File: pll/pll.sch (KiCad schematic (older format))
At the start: 24 parts, among them SW1 SW_DIP_x05, U1 NE555, U2 74HC393, U3 74HC86, U4 LM7805, U5 NE555

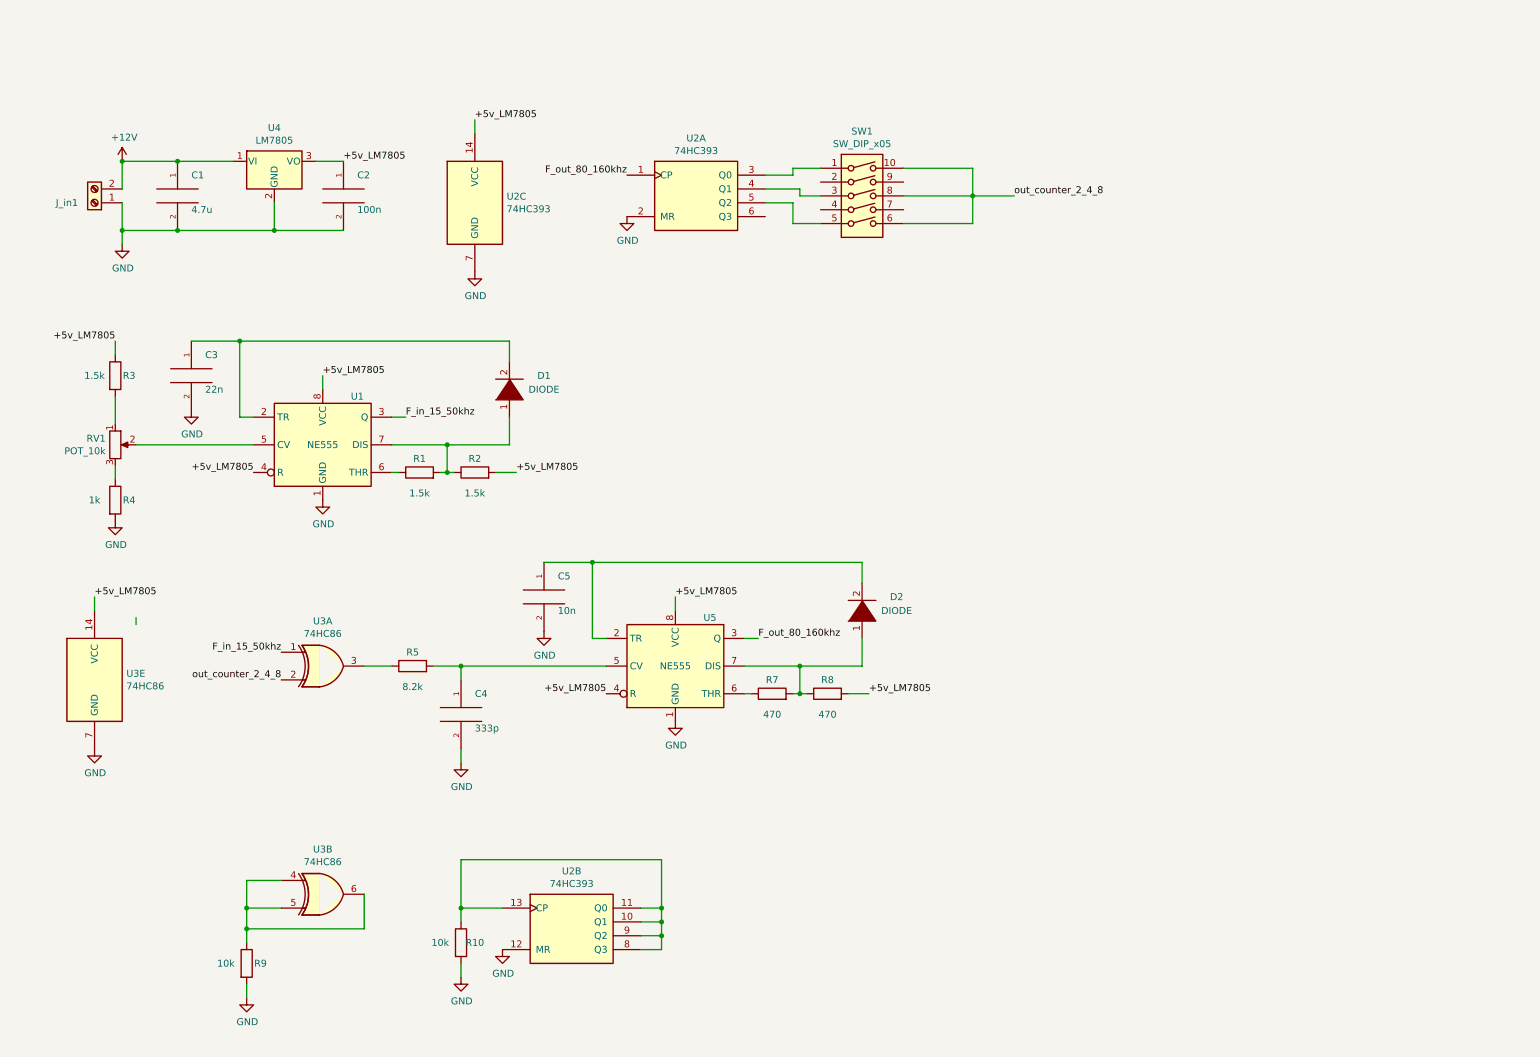
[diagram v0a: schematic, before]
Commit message: Update pll
Signed-off-by: Felipe Leon <fglfgl27@gmail.com>
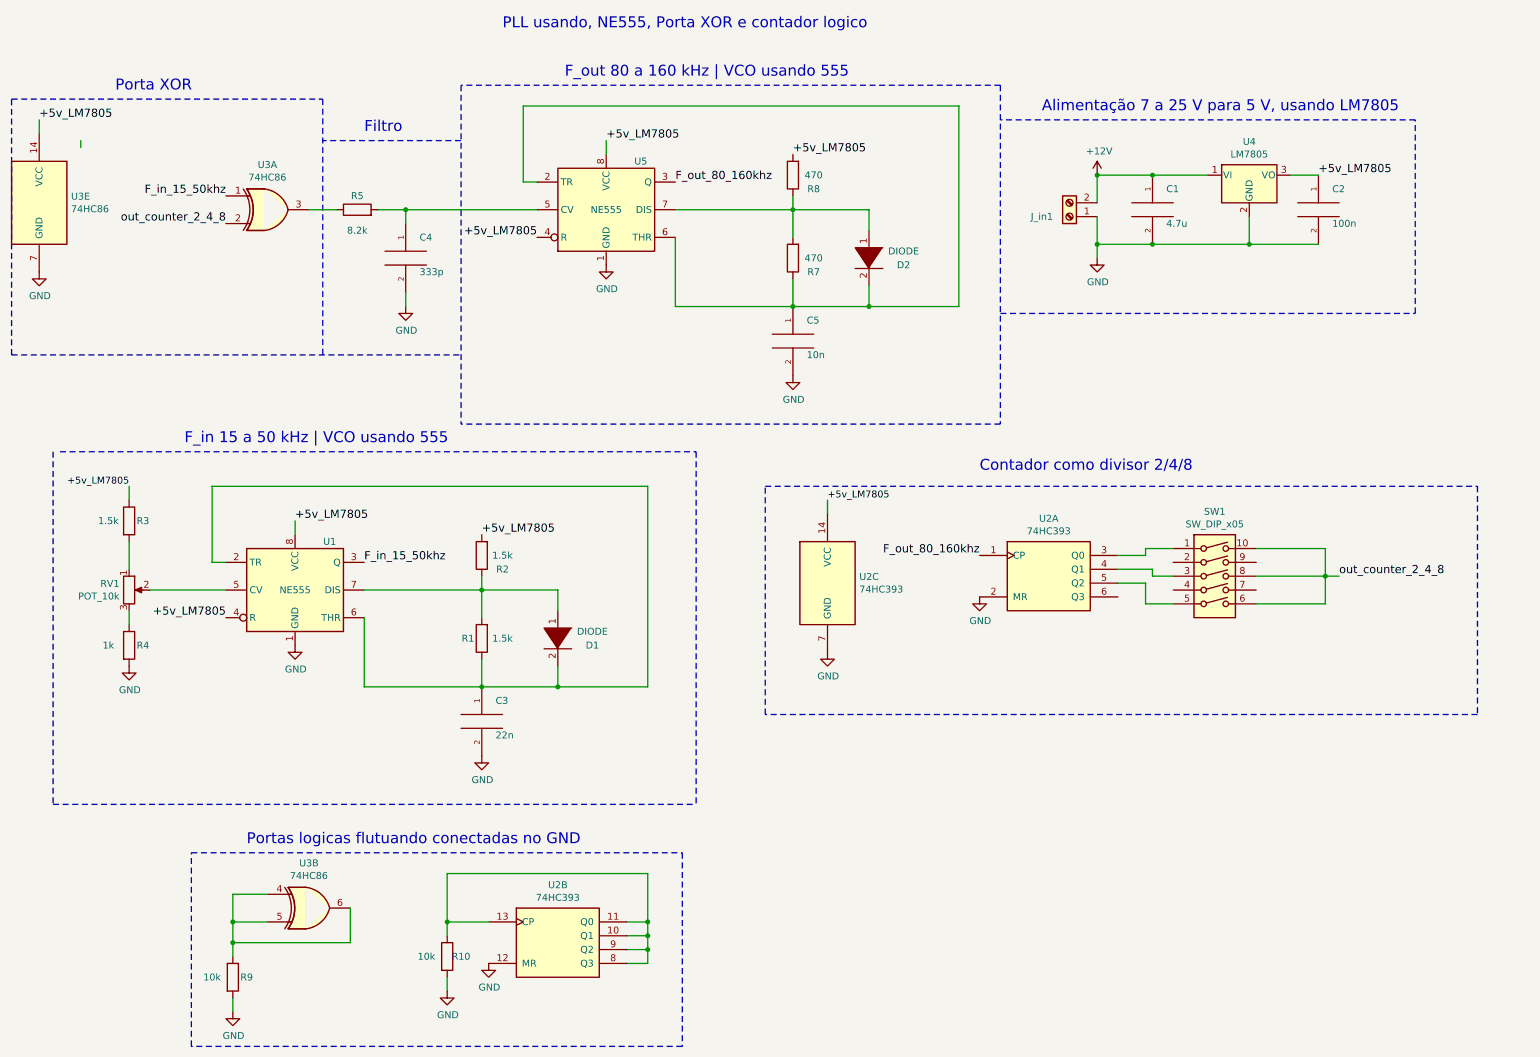
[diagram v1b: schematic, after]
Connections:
- net at C3.1, D1.2 (A), U1.2 (TR): now also R1.1, U1.6 (THR)
- net at C5.1, D2.2 (A), U5.2 (TR): now also R7.1, U5.6 (THR)
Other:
- note added: "Alimentação 7 a 25 V para 5 V, usando LM7805"
- note added: "Contador como divisor 2/4/8"
- note added: "F_in 15 a 50 kHz | VCO usando 555"
- note added: "F_out 80 a 160 kHz | VCO usando 555"
- note added: "Filtro"
- note added: "PLL usando, NE555, Porta XOR e contador logico"
- note added: "Porta XOR"
- note added: "Portas logicas flutuando conectadas no GND"
- moved on the sheet: C1, C2, C4, C5, D2, J_in1, R10, R3, R4, R5, R7, R8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
